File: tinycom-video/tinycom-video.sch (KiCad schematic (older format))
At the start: 42 parts, among them J1 MICRO_SD_HINGE, P1 CONN_02X10, P2 CONN_02X10, P4 USB_OTG, U1 SY8008BAAC, U2 AXP209, U3 SY8008BAAC, U4 RTL8188, U5 rainsun-antenna

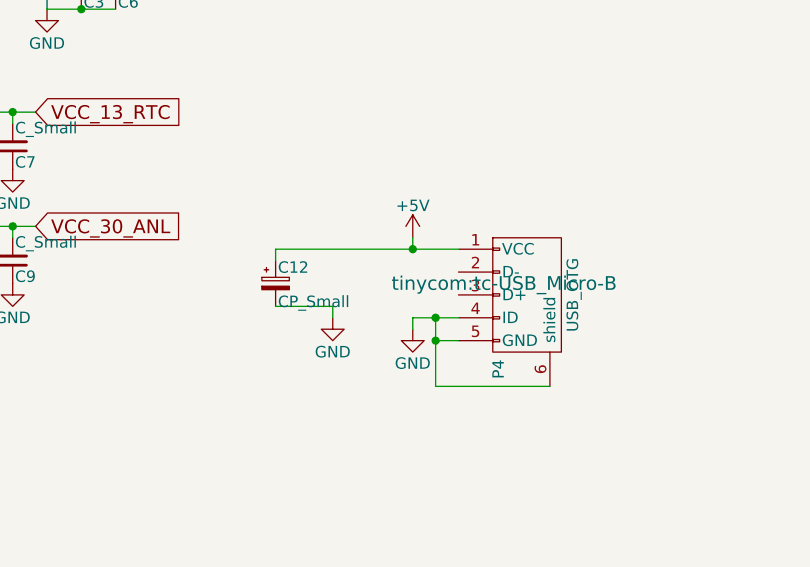
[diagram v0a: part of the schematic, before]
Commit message: vid usb
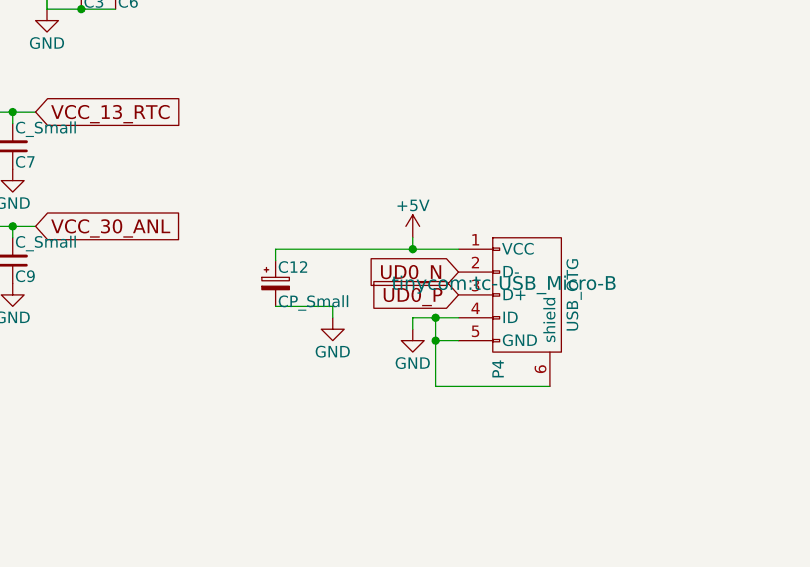
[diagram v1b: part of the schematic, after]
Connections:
- net UD0_N: now also P4.2 (D-)
- net UD0_P: now also P4.3 (D+)
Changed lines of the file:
@@
 	1150 8100 1750 8100
 Connection ~ 1750 8100
+Text GLabel 5450 4450 0    60   Input ~ 0
+UD0_P
+Text GLabel 5450 4350 0    60   Input ~ 0
+UD0_N
 $EndSCHEMATC
